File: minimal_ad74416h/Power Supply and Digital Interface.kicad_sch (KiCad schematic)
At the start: 89 parts, among them T1 ZA9644-AED, U1 MAX17570FATA+, U4 ADP1031ACPZ-2-R7, U5 ADUM1252AUA+, U6 ADUM1252AUA+, U7 ADUM1252AUA+

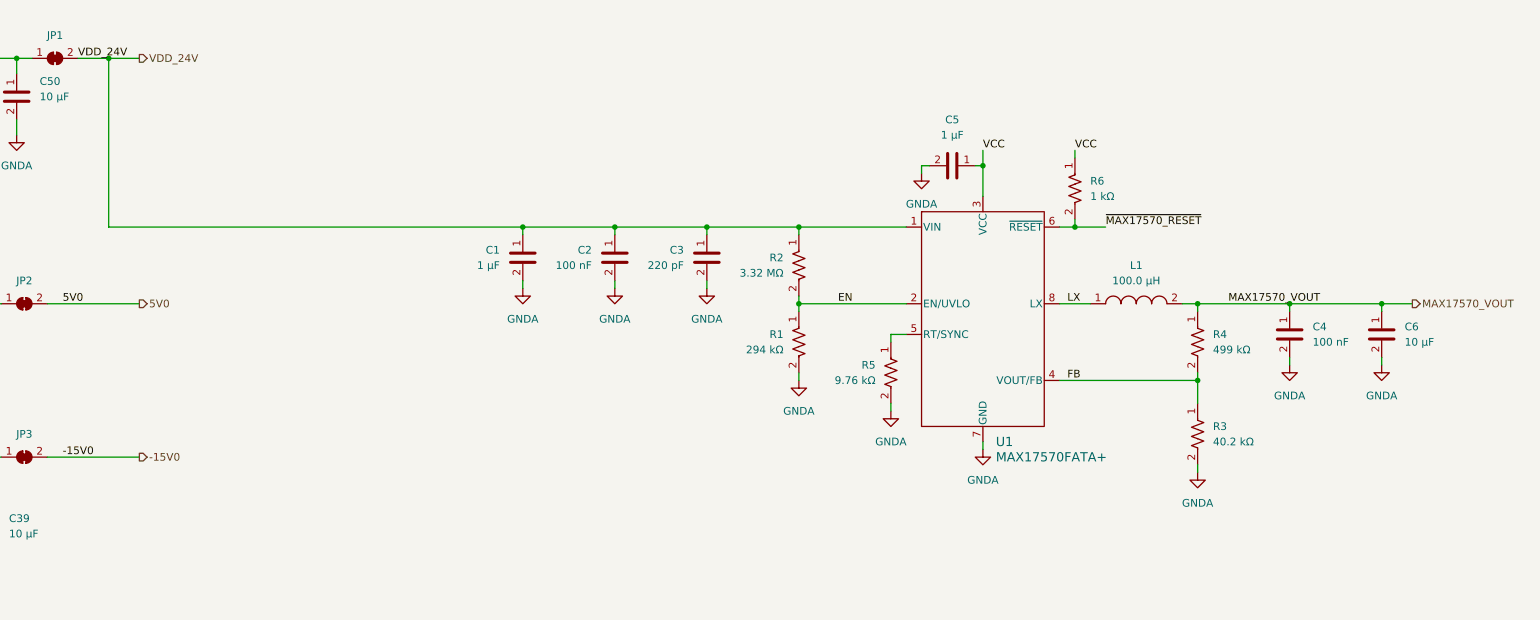
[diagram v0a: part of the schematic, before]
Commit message: backup
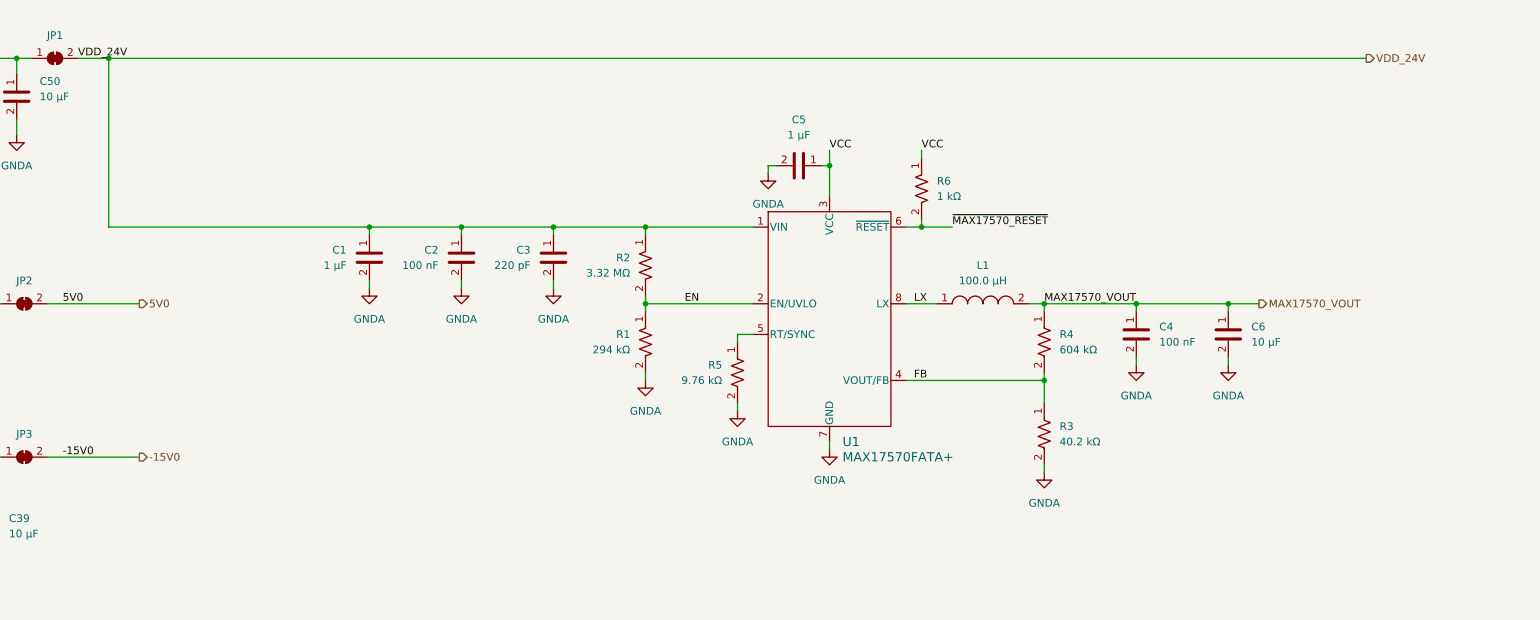
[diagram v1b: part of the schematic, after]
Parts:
- L1: footprint inductor_footprints:74404054 -> inductor_footprints:74404032; symbol INDUCTORS_74404054_DATA_BASE:L_74404054101 -> INDUCTORS_74404032_DATA_BASE:L_74404032101; MPN 74404054101 -> 74404032101; Maximum DC Current (A) 0.7 -> 0.3; Maximum DC Resistance (Ω) 0.560 -> 1.900; Series 74404054 -> 74404032; Symbol Name L_74404054101 -> L_74404032101; Trustedparts Search https://www.trustedparts.com/en/search/74404054101 -> https://www.trustedparts.com/en/search/74404032101
- R4: value 499 kΩ -> 604 kΩ; symbol RESISTORS_ERJ-2RKF_DATA_BASE:R_ERJ-2RKF4993X -> RESISTORS_ERJ-2RKF_DATA_BASE:R_ERJ-2RKF6043X; MPN ERJ-2RKF4993X -> ERJ-2RKF6043X; Symbol Name R_ERJ-2RKF4993X -> R_ERJ-2RKF6043X; Trustedparts Search https://www.trustedparts.com/en/search/ERJ-2RKF4993X -> https://www.trustedparts.com/en/search/ERJ-2RKF6043X
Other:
- moved on the sheet: C1, C2, C3, C4, C5, C6, L1, R1, R2, R3, R4, R5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
